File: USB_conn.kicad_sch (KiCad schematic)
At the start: 7 parts, among them P1 USB_C_Plug_USB2.0

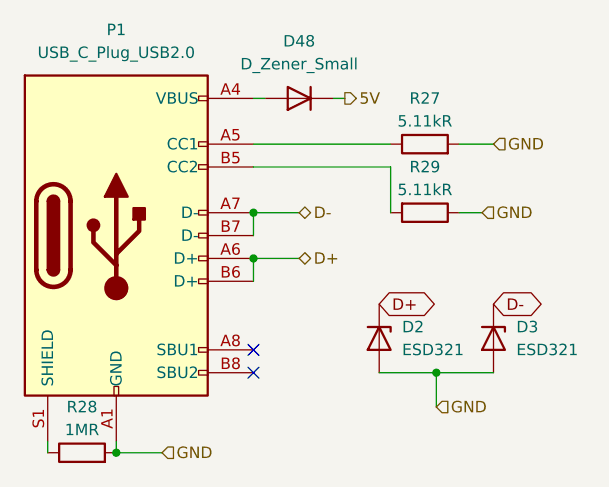
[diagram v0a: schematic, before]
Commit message: update BOM + add big capas (do not take DNP into account)
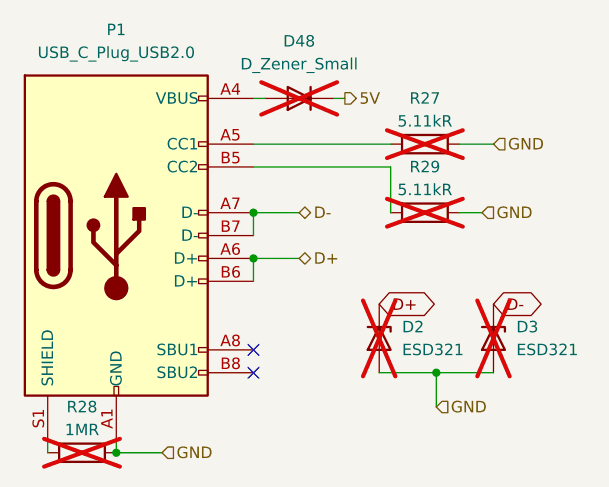
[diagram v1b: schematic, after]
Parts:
- D2, D3, D48, R27, R28, R29: now not fitted
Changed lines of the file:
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@@
 		(in_bom yes)
 		(on_board yes)
-		(dnp no)
+		(dnp yes)
 		(fields_autoplaced yes)
 		(property "Reference" "D48"
@@
 		(in_bom yes)
 		(on_board yes)
-		(dnp no)
+		(dnp yes)
 		(fields_autoplaced yes)
 		(property "Reference" "R29"
@@
 		(in_bom yes)
 		(on_board yes)
-		(dnp no)
+		(dnp yes)
 		(fields_autoplaced yes)
 		(property "Reference" "R27"
@@
 		(in_bom yes)
 		(on_board yes)
-		(dnp no)
+		(dnp yes)
 		(fields_autoplaced yes)
 		(property "Reference" "D2"
@@
 		(in_bom yes)
 		(on_board yes)
-		(dnp no)
+		(dnp yes)
 		(fields_autoplaced yes)
 		(property "Reference" "D3"
@@
 		(in_bom yes)
 		(on_board yes)
-		(dnp no)
+		(dnp yes)
 		(fields_autoplaced yes)
 		(property "Reference" "R28"

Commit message: fix DNP (was just for checking what was to be bought)
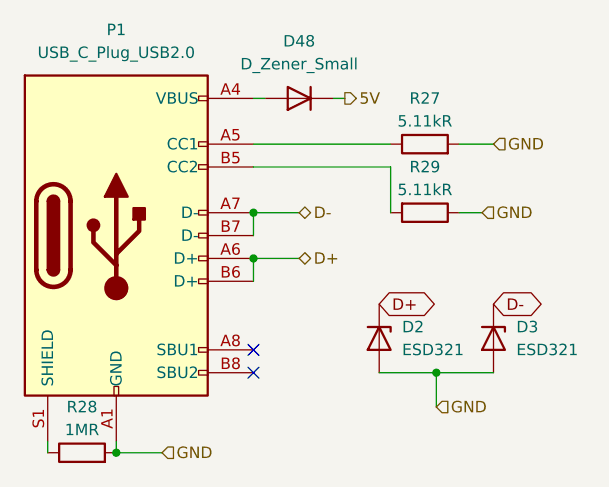
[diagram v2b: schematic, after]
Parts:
- D2, D3, D48, R27, R28, R29: now fitted
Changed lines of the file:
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@@
 		(in_bom yes)
 		(on_board yes)
-		(dnp yes)
+		(dnp no)
 		(fields_autoplaced yes)
 		(property "Reference" "D48"
@@
 		(in_bom yes)
 		(on_board yes)
-		(dnp yes)
+		(dnp no)
 		(fields_autoplaced yes)
 		(property "Reference" "R29"
@@
 		(in_bom yes)
 		(on_board yes)
-		(dnp yes)
+		(dnp no)
 		(fields_autoplaced yes)
 		(property "Reference" "R27"
@@
 		(in_bom yes)
 		(on_board yes)
-		(dnp yes)
+		(dnp no)
 		(fields_autoplaced yes)
 		(property "Reference" "D2"
@@
 		(in_bom yes)
 		(on_board yes)
-		(dnp yes)
+		(dnp no)
 		(fields_autoplaced yes)
 		(property "Reference" "D3"
@@
 		(in_bom yes)
 		(on_board yes)
-		(dnp yes)
+		(dnp no)
 		(fields_autoplaced yes)
 		(property "Reference" "R28"
